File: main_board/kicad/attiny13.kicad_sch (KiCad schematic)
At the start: 6 parts

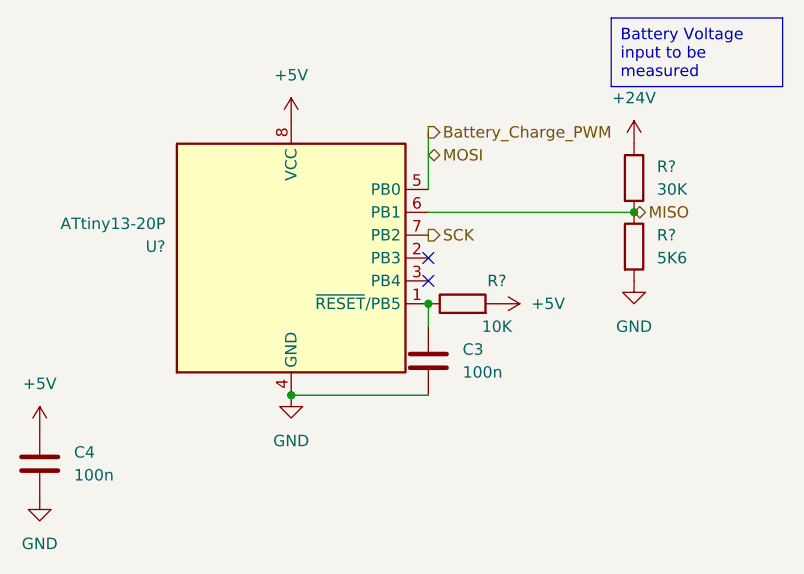
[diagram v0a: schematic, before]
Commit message: updated to post review state
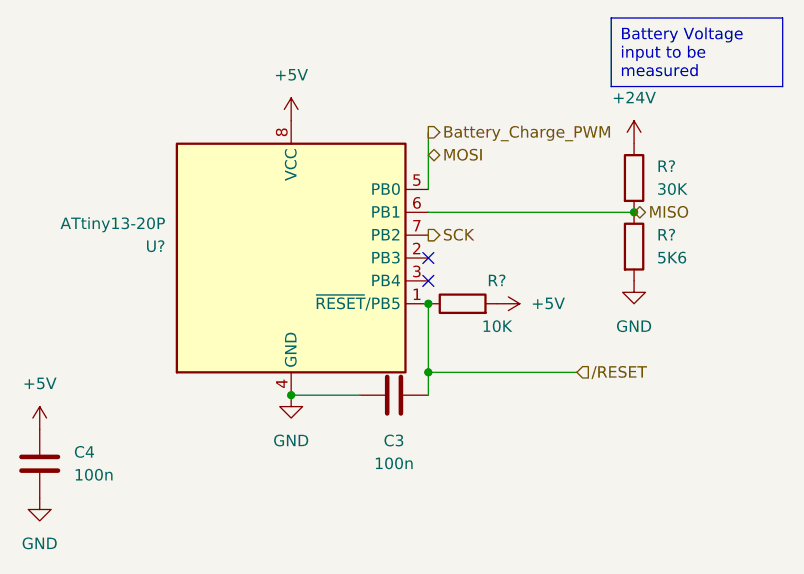
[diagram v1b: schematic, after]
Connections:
- net GND: now also C3.1; no longer C3.2
- net /RESET: now reaches R?.1, U?.1 (~{RESET}/PB5)
- net /RESET: now also C3.2; no longer C3.1
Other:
- moved on the sheet: C3
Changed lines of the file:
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@@
 (kicad_sch (version 20230121) (generator eeschema)
   (paper "A4")
+  (junction (at 149.86 111.76) (diameter 0) (color 0 0 0 0)
+  )
+  (junction (at 134.62 114.3) (diameter 0) (color 0 0 0 0)
+  )
   (junction (at 149.86 104.14) (diameter 0) (color 0 0 0 0)
   )
   (junction (at 172.72 93.98) (diameter 0) (color 0 0 0 0)
   )
-  (junction (at 134.62 114.3) (diameter 0) (color 0 0 0 0)
-  )
   (no_connect (at 149.86 101.6))
   (no_connect (at 149.86 99.06))
+  (wire (pts (xy 149.86 111.76) (xy 149.86 114.3))
+    (stroke (width 0) (type default))
+  )
   (wire (pts (xy 149.86 85.09) (xy 149.86 91.44))
+    (stroke (width 0) (type default))
+  )
+  (wire (pts (xy 149.86 111.76) (xy 166.37 111.76))
     (stroke (width 0) (type default))
   )
@@
     (stroke (width 0) (type default))
   )
-  (wire (pts (xy 134.62 114.3) (xy 149.86 114.3))
+  (wire (pts (xy 134.62 114.3) (xy 142.24 114.3))
     (stroke (width 0) (type default))
   )
-  (wire (pts (xy 149.86 106.68) (xy 149.86 104.14))
+  (wire (pts (xy 149.86 104.14) (xy 149.86 111.76))
     (stroke (width 0) (type default))
   )
@@
     (effects (font (size 1.27 1.27)) (justify left))
   )
-  (symbol (lib_id "Device:C") (at 149.86 110.49 0) (unit 1)
-    (in_bom yes) (on_board yes) (dnp no) (fields_autoplaced)
-    (property "Reference" "C3" (at 153.67 109.22 0)
-      (effects (font (size 1.27 1.27)) (justify left))
+  (hierarchical_label "{slash}RESET" (shape input) (at 166.37 111.76 0) (fields_autoplaced)
+    (effects (font (size 1.27 1.27)) (justify left))
+  )
+  (symbol (lib_id "Device:C") (at 146.05 114.3 90) (unit 1)
+    (in_bom yes) (on_board yes) (dnp no)
+    (property "Reference" "C3" (at 146.05 119.38 90)
+      (effects (font (size 1.27 1.27)))
     )
-    (property "Value" "100n" (at 153.67 111.76 0)
-      (effects (font (size 1.27 1.27)) (justify left))
+    (property "Value" "100n" (at 146.05 121.92 90)
+      (effects (font (size 1.27 1.27)))
     )
-    (property "Footprint" "" (at 150.8252 114.3 0)
+    (property "Footprint" "" (at 149.86 113.3348 0)
       (effects (font (size 1.27 1.27)) hide)
     )
-    (property "Datasheet" "~" (at 149.86 110.49 0)
+    (property "Datasheet" "~" (at 146.05 114.3 0)
       (effects (font (size 1.27 1.27)) hide)
     )

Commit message: added footprints
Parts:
- C3, C4: footprint (none) -> Capacitor_THT:C_Disc_D3.0mm_W1.6mm_P2.50mm
- R? (x3): footprint (none) -> Resistor_THT:R_Axial_DIN0207_L6.3mm_D2.5mm_P7.62mm_Horizontal
- U?: footprint Package_DIP:DIP-8_W7.62mm -> Package_DIP:DIP-8_W7.62mm_LongPads
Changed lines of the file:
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@@
       (effects (font (size 1.27 1.27)))
     )
-    (property "Footprint" "" (at 149.86 113.3348 0)
+    (property "Footprint" "Capacitor_THT:C_Disc_D3.0mm_W1.6mm_P2.50mm" (at 149.86 113.3348 0)
       (effects (font (size 1.27 1.27)) hide)
     )
@@
       (effects (font (size 1.27 1.27)) (justify left))
     )
-    (property "Footprint" "" (at 170.942 97.79 90)
+    (property "Footprint" "Resistor_THT:R_Axial_DIN0207_L6.3mm_D2.5mm_P7.62mm_Horizontal" (at 170.942 97.79 90)
       (effects (font (size 1.27 1.27)) hide)
     )
@@
       (effects (font (size 1.27 1.27)) (justify left))
     )
-    (property "Footprint" "" (at 107.6452 125.73 0)
+    (property "Footprint" "Capacitor_THT:C_Disc_D3.0mm_W1.6mm_P2.50mm" (at 107.6452 125.73 0)
       (effects (font (size 1.27 1.27)) hide)
     )
@@
       (effects (font (size 1.27 1.27)))
     )
-    (property "Footprint" "" (at 153.67 105.918 90)
+    (property "Footprint" "Resistor_THT:R_Axial_DIN0207_L6.3mm_D2.5mm_P7.62mm_Horizontal" (at 153.67 105.918 90)
       (effects (font (size 1.27 1.27)) hide)
     )
@@
       (effects (font (size 1.27 1.27)) (justify right))
     )
-    (property "Footprint" "Package_DIP:DIP-8_W7.62mm" (at 134.62 99.06 0)
+    (property "Footprint" "Package_DIP:DIP-8_W7.62mm_LongPads" (at 134.62 99.06 0)
       (effects (font (size 1.27 1.27) italic) hide)
     )
@@
       (effects (font (size 1.27 1.27)) (justify left))
     )
-    (property "Footprint" "" (at 170.942 90.17 90)
+    (property "Footprint" "Resistor_THT:R_Axial_DIN0207_L6.3mm_D2.5mm_P7.62mm_Horizontal" (at 170.942 90.17 90)
       (effects (font (size 1.27 1.27)) hide)
     )
